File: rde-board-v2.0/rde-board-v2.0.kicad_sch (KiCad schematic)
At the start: 19 parts, among them J1 RPI conn, J2 Mouse / Joy 1, J3 Joy 2, U1 ULN2003A, U2 ULN2003A

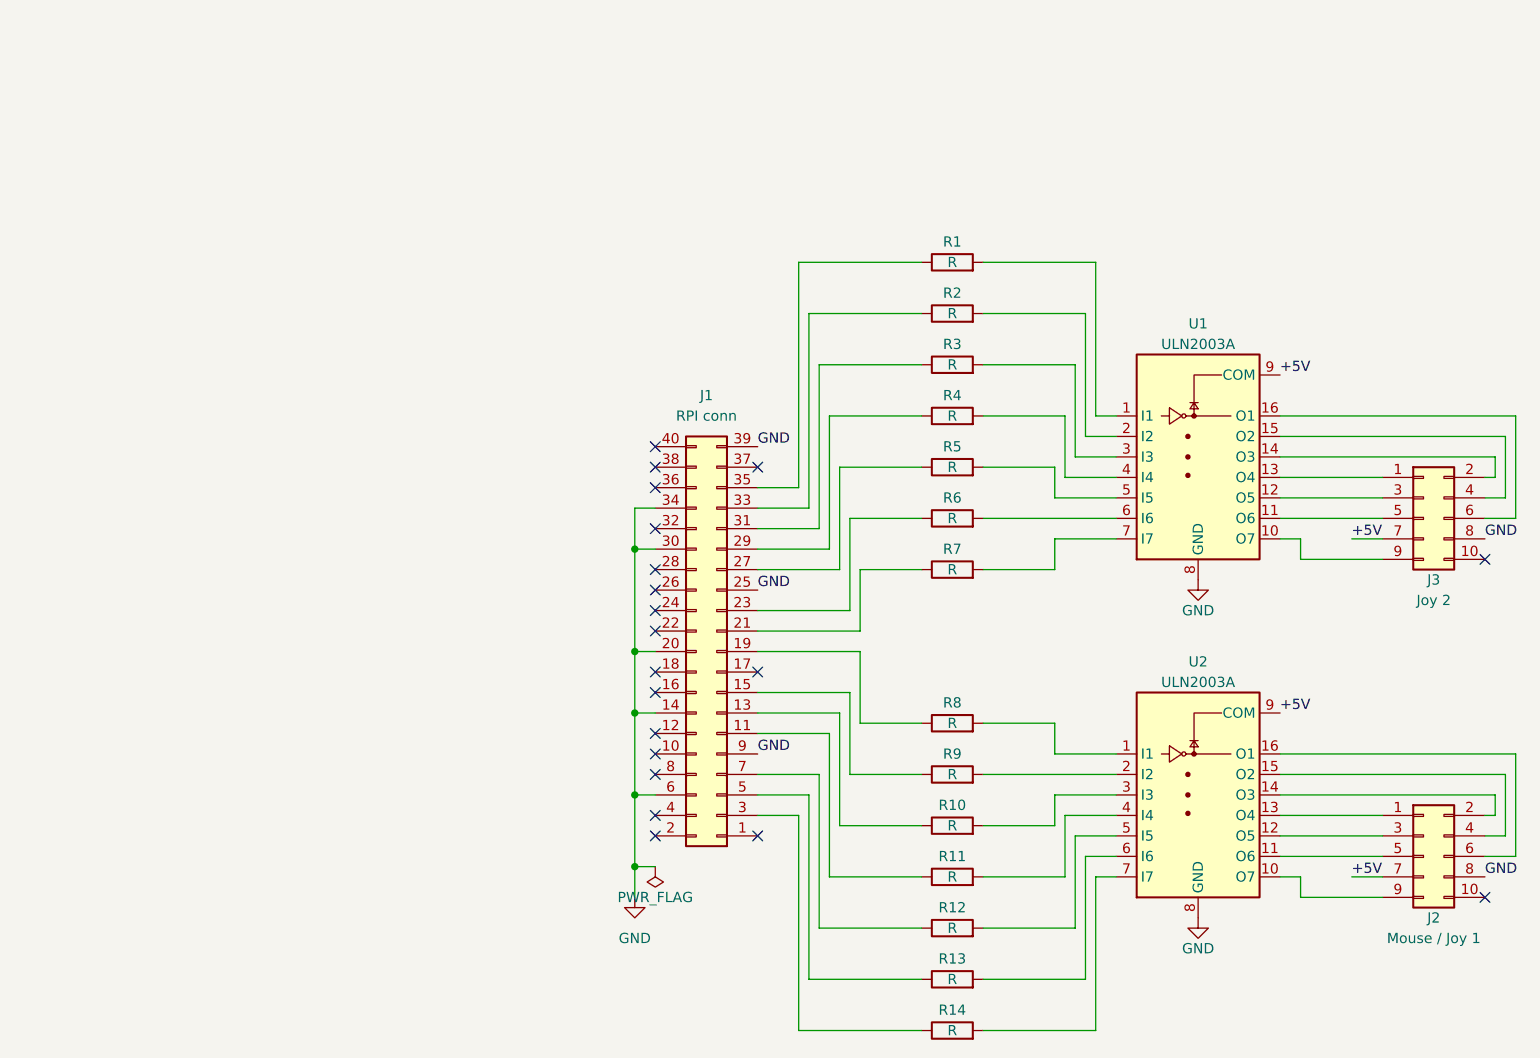
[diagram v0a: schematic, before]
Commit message: Update rde-board
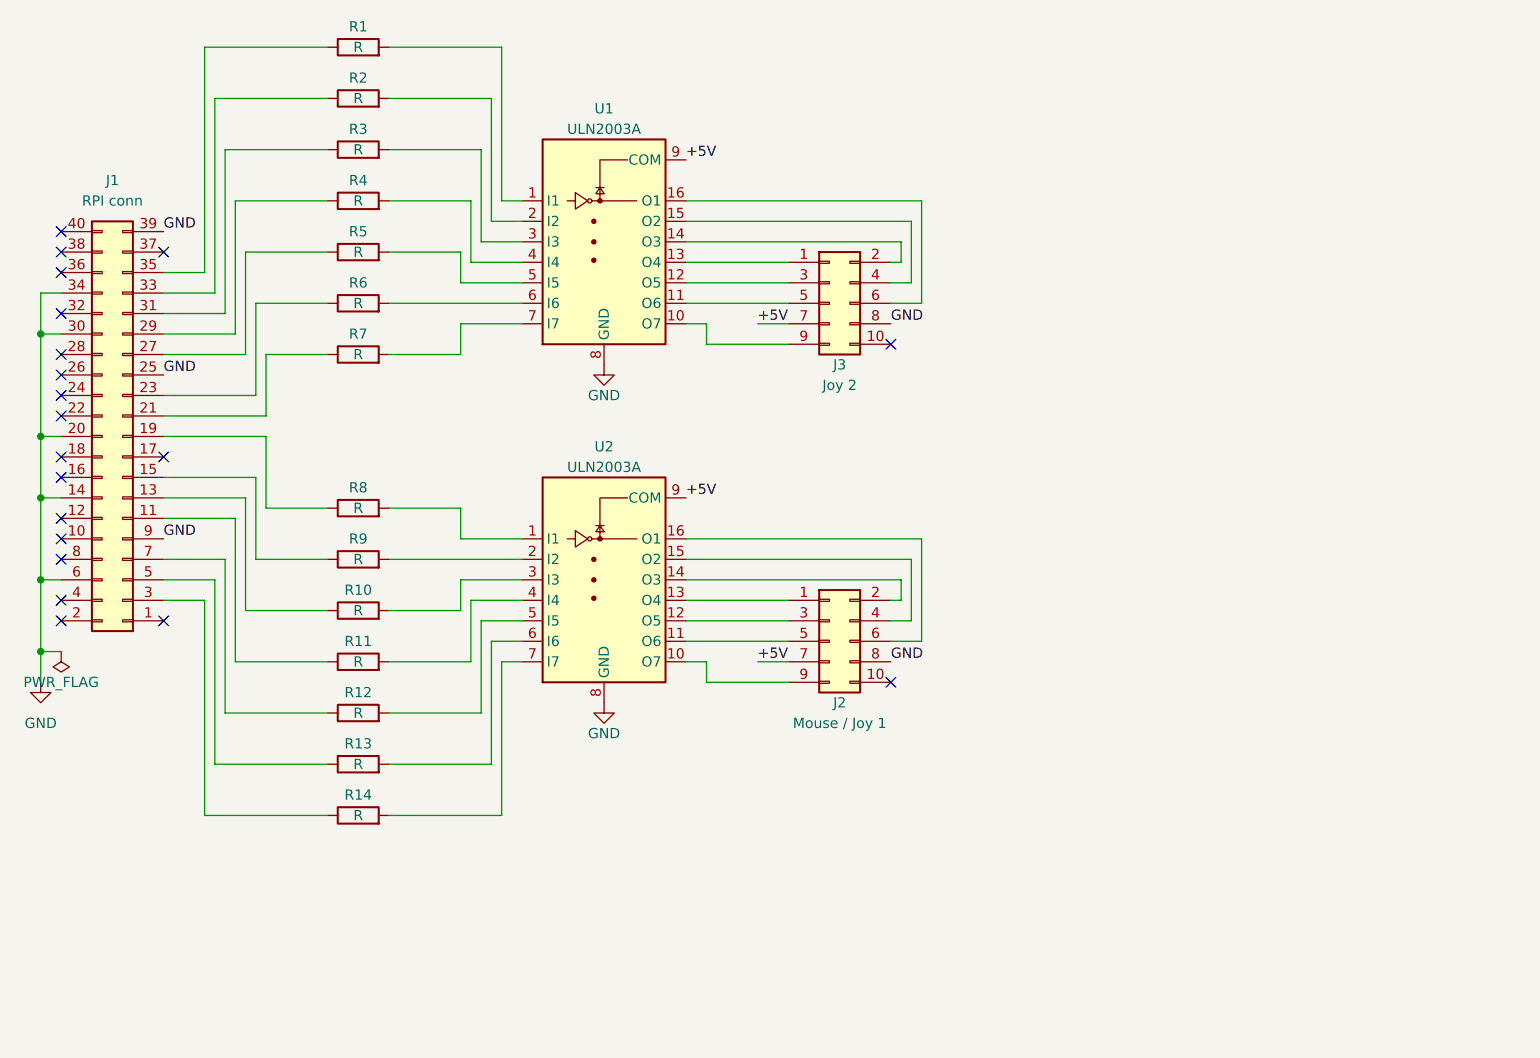
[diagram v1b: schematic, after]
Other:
- title: (none) -> RetroDevEm
- moved on the sheet: J1, J2, J3, R1, R10, R11, R12, R13, R14, R2, R3, R4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
